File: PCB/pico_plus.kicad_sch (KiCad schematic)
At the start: 50 parts, among them J1 USB_C_Receptacle_USB2.0_16P, SW1 SW_Push, SW2 SW_Push, SW3 SW_Push, U1 RP2350_60QFN, U2 TPS7A20xxxDQN, U3 W25Q128JVP, U4 APS6404L-3SQR-ZR, Y1 ABM8-272-T3

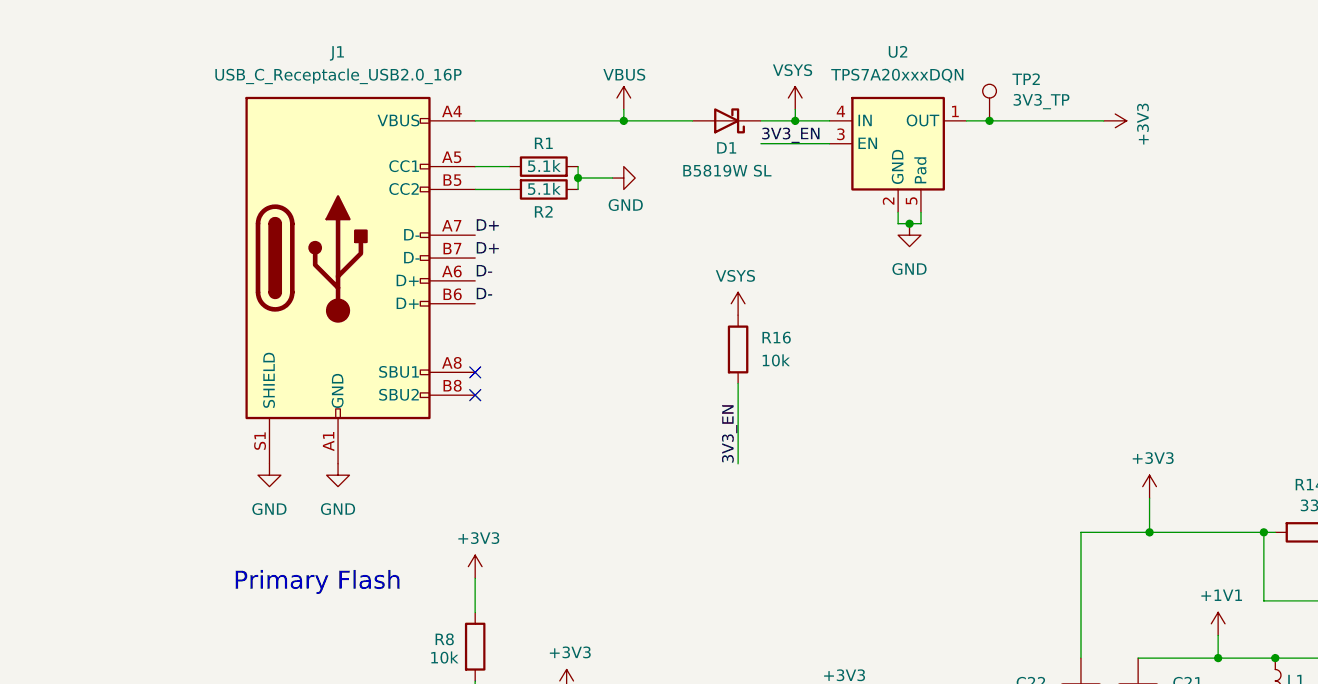
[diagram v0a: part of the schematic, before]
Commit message: finish up pcb + bom
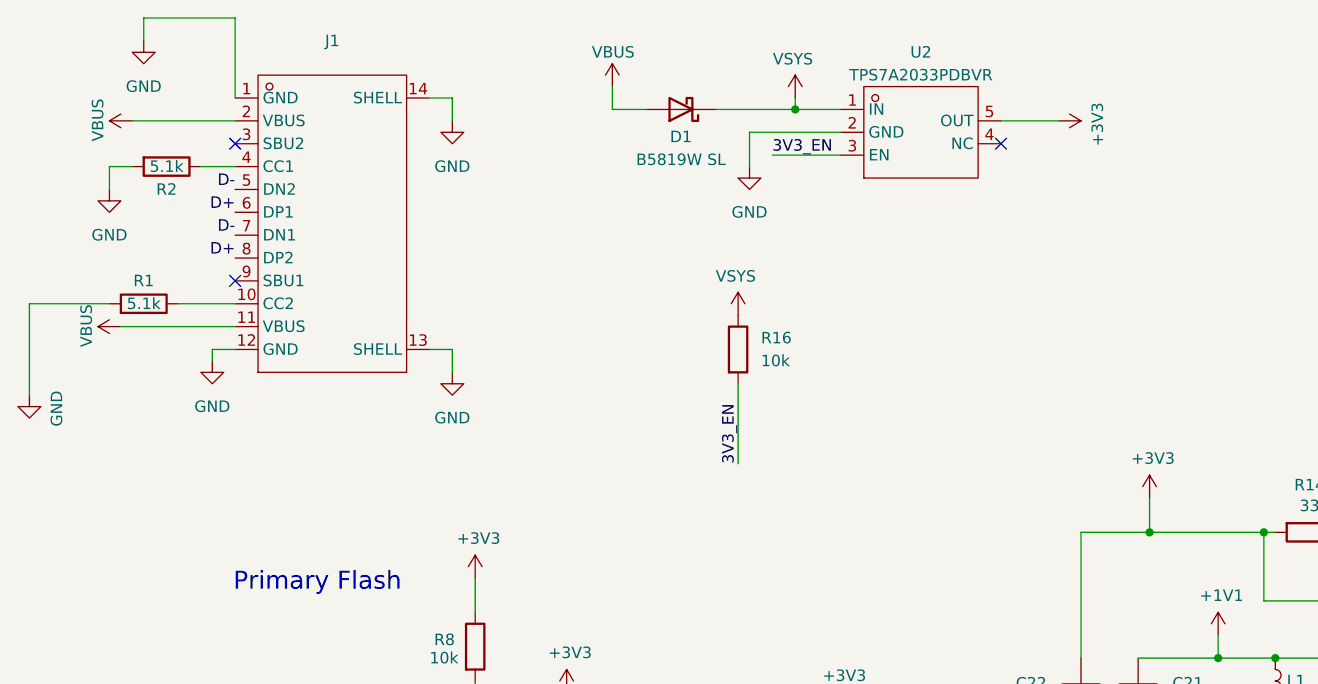
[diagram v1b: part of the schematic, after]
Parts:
- removed J1: USB_C_Receptacle_USB2.0_16P, Connector_USB:USB_C_Receptacle_GCT_USB4105-xx-A_16P_TopMnt_Horizontal, symbol Connector:USB_C_Receptacle_USB2.0_16P
- removed TP2: 3V3_TP, TestPoint:TestPoint_Pad_D1.0mm, symbol Connector:TestPoint
- removed U2: TPS7A20xxxDQN, Package_SON:Texas_X2SON-4_1x1mm_P0.65mm, symbol Regulator_Linear:TPS7A20xxxDQN
- added J1: ~, Components:USB-C-SMD_TYPE-C-6PIN-2MD-073, symbol USB_C:TYPE-C 16PIN 2MD(073)
- added U2: TPS7A2033PDBVR, Components:SOT-23-5_L2.9-W1.6-P0.95-LS2.8-BR, symbol Pico:TPS7A2033PDBVR
- C10, C19, C20, C3, C4: footprint Capacitor_SMD:C_0201_0603Metric -> Capacitor_SMD:C_0402_1005Metric
- R1, R11, R13, R14, R15, R16, R2, R5, R6, R7, R8: footprint Resistor_SMD:R_0201_0603Metric -> Resistor_SMD:R_0402_1005Metric
- R12: footprint Resistor_SMD:R_0201_0603Metric -> Resistor_SMD:R_0603_1608Metric
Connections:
- net +3V3: now also U2.5 (OUT)
- net 3V3_EN: now also U2.3 (EN)
- net D+: now also J1.6 (DP1), J1.8 (DP2)
- net D-: now also J1.5 (DN2), J1.7 (DN1)
- net GND: now also R2.2, J1.1 (GND), J1.12 (GND), J1.13 (SHELL), J1.14 (SHELL), U2.2 (GND); no longer R2.1
- net VBUS: now also J1.11 (VBUS), J1.2 (VBUS)
- net VSYS: now also U2.1 (IN)
- net at R1.1: now also J1.10 (CC2)
- new net: J1.4 (CC1), R2.1
- no-connect marks 2 -> 3
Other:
- moved on the sheet: D1, R1, R2
